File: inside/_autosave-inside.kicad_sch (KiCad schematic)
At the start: 6 parts, among them J1 Barrel_Jack, M1 Stepper_Motor_bipolar, M2 Stepper_Motor_bipolar, U2 ESP32-WROOM-32

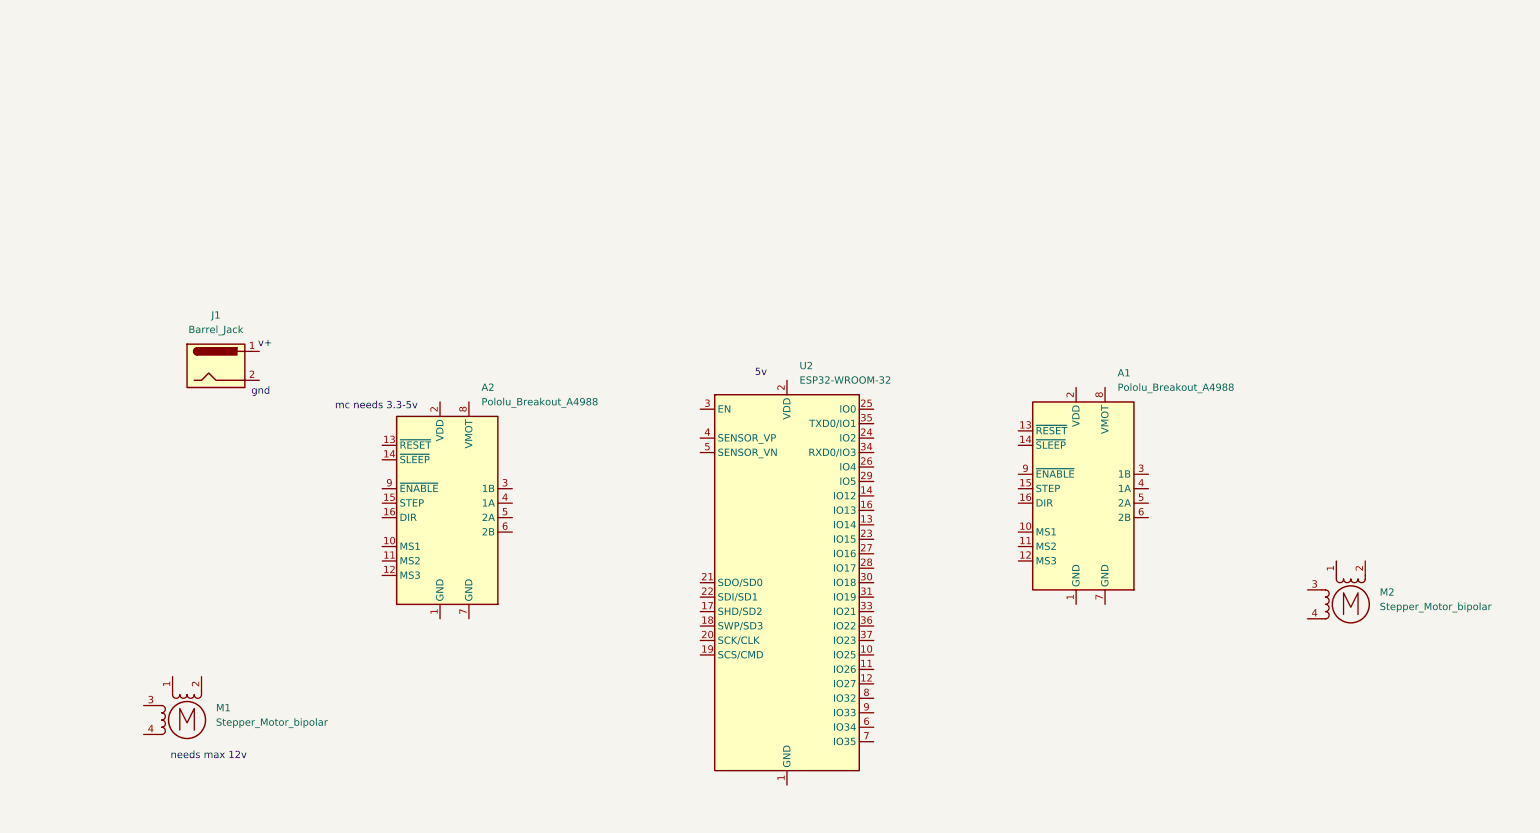
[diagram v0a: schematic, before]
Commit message: day 2 and 3
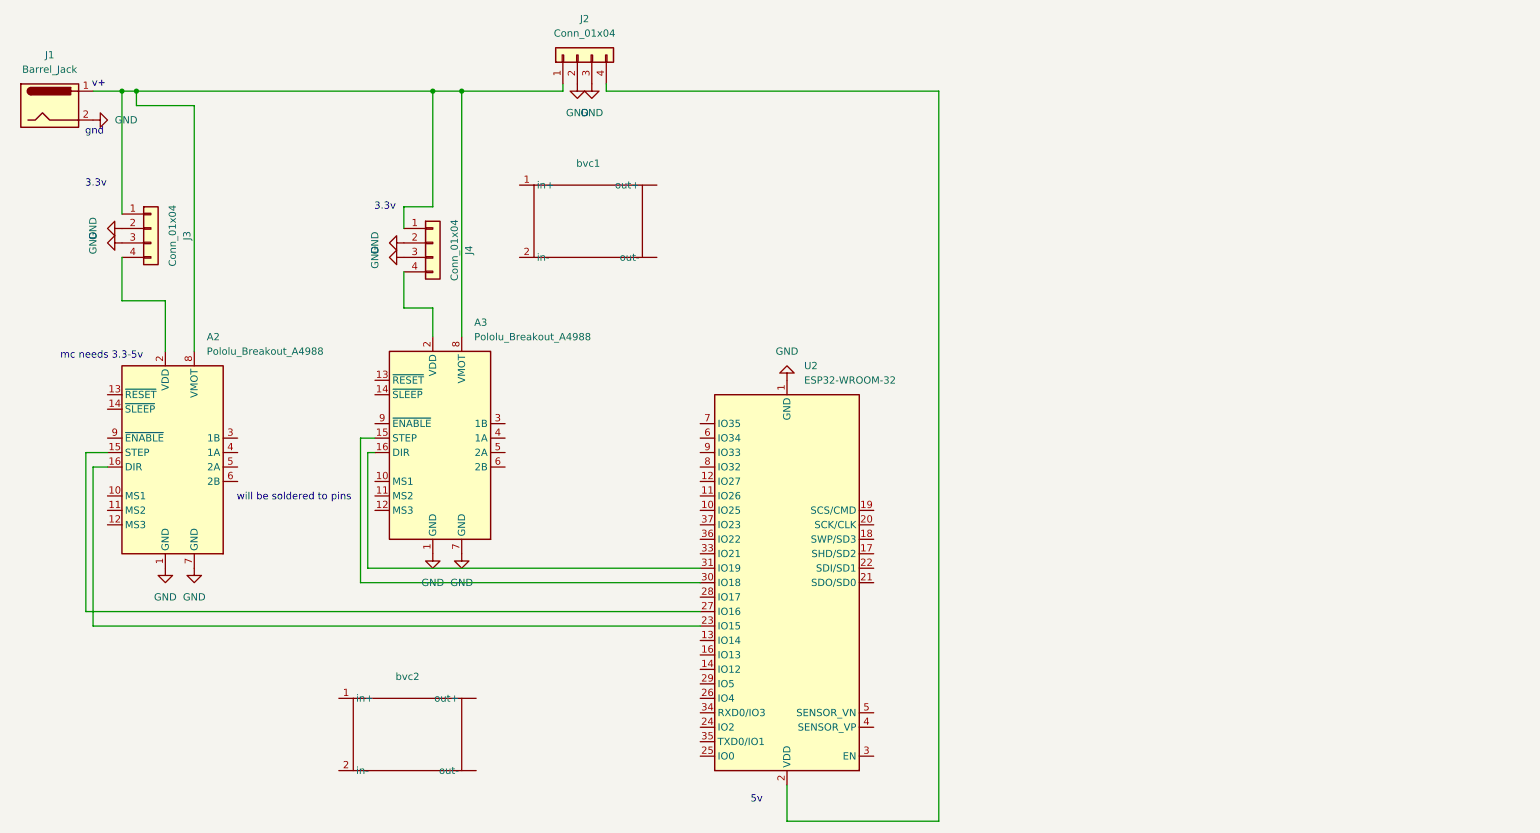
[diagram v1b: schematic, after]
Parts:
- removed A1: Pololu_Breakout_A4988, Module:Pololu_Breakout-16_15.2x20.3mm, symbol Driver_Motor:Pololu_Breakout_A4988
- removed M1, M2: Stepper_Motor_bipolar, symbol Motor:Stepper_Motor_bipolar
- added A3: Pololu_Breakout_A4988, Module:Pololu_Breakout-16_15.2x20.3mm, symbol Driver_Motor:Pololu_Breakout_A4988
- added J2, J3, J4: Conn_01x04, Converter_DCDC:buck voltage converter, symbol Connector_Generic:Conn_01x04
- added bvc1, bvc2: ~, symbol Converter_DCDC:buck_voltage_converter
- J1: footprint (none) -> Connector_BarrelJack:BarrelJack_Horizontal
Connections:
- net at J1.1: now also A2.8 (VMOT), A3.8 (VMOT), J2.1 (Pin_1), J3.1 (Pin_1), J4.1 (Pin_1)
- net GND: now reaches J1.2
- net GND: now also A2.1 (GND), A2.7 (GND), U2.1 (GND), U2.15 (GND), U2.38 (GND), U2.39 (GND), A3.1 (GND), A3.7 (GND), J2.2 (Pin_2), J2.3 (Pin_3), J3.2 (Pin_2), J3.3 (Pin_3), J4.2 (Pin_2), J4.3 (Pin_3)
- net at A2.15 (STEP): now also U2.27 (IO16)
- net at A2.16 (DIR): now also U2.23 (IO15)
- net at A2.2 (VDD): now also J3.4 (Pin_4)
- net at U2.2 (VDD): now also J2.4 (Pin_4)
- net at U2.30 (IO18): now also A3.15 (STEP)
- net at U2.31 (IO19): now also A3.16 (DIR)
- new net: A3.2 (VDD), J4.4 (Pin_4)
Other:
- note added: "3.3v"
- note added: "will be soldered to pins"
- note removed: "needs max 12v"
- moved on the sheet: A2, J1, U2
